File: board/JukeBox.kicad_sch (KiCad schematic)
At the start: 44 parts, among them J1 USB_C_Receptacle_USB2.0, J2 Conn_01x02, J3 Conn_01x04, J4 Conn_01x03, J5 Conn_01x08, SW1 SW_SPST, SW10 SW_SPST, SW11 SW_SPST, SW12 SW_SPST, SW2 SW_SPST, SW3 SW_SPST, SW4 SW_SPST, SW5 SW_SPST, SW6 SW_SPST, SW7 SW_SPST, SW8 SW_SPST, SW9 SW_SPST, U1 ATmega8U2-A, Y1 16MHz

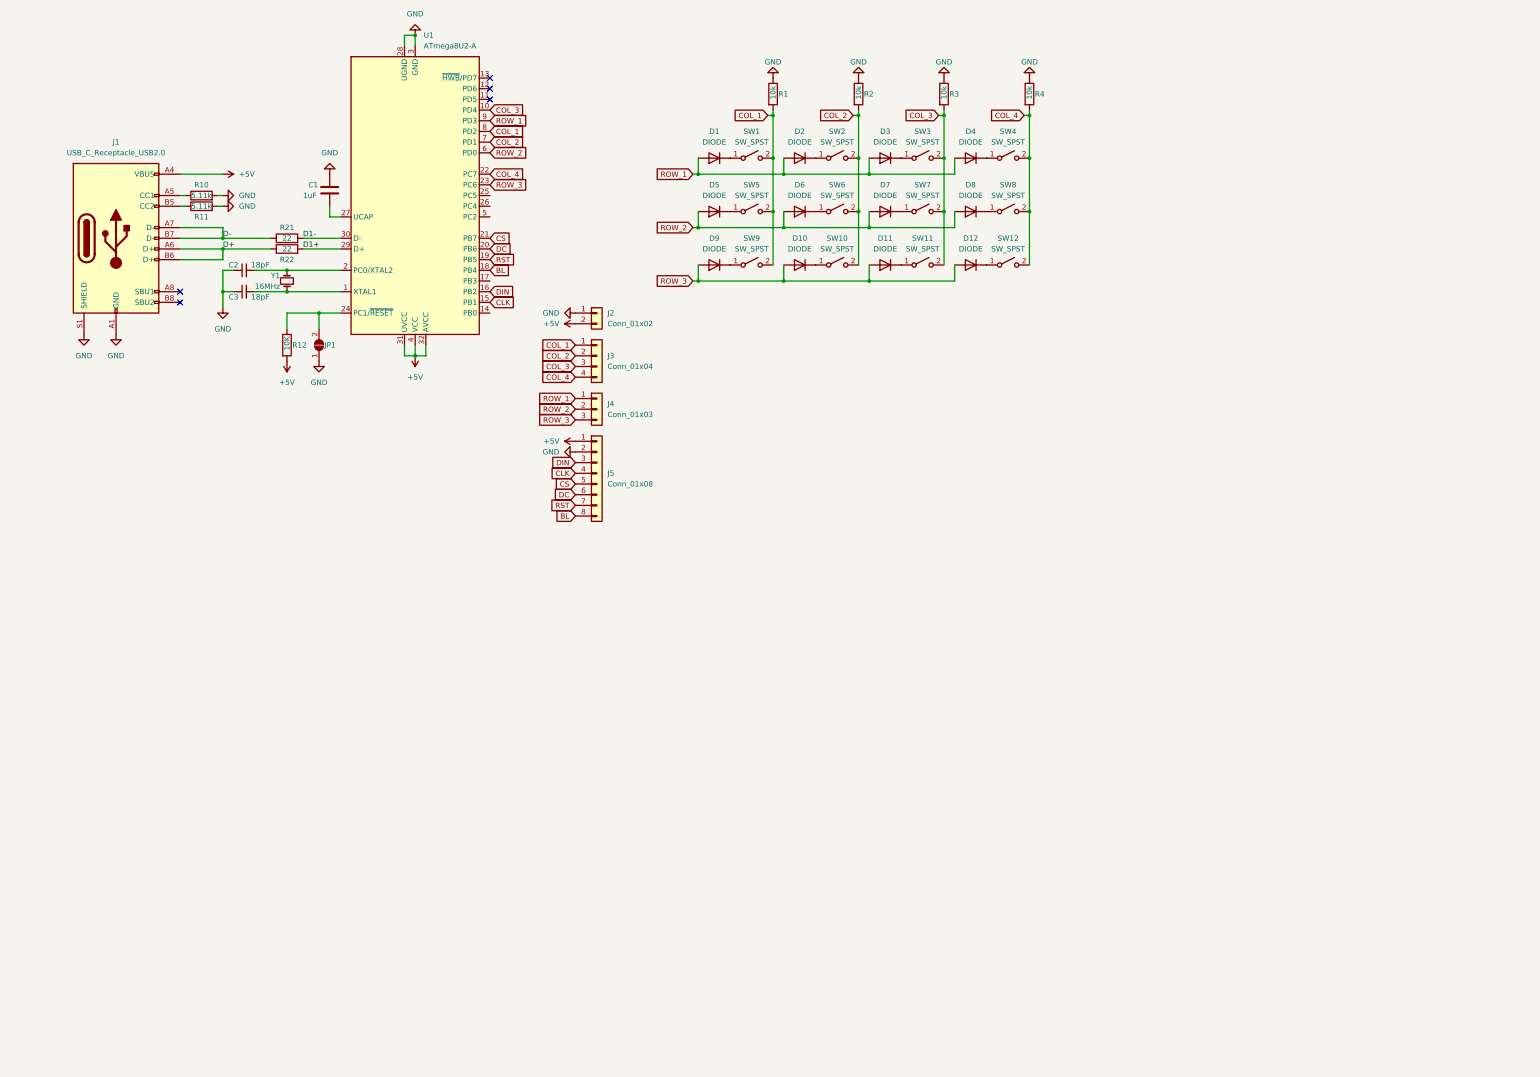
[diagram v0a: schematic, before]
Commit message: import rp2040 minimal kicad project
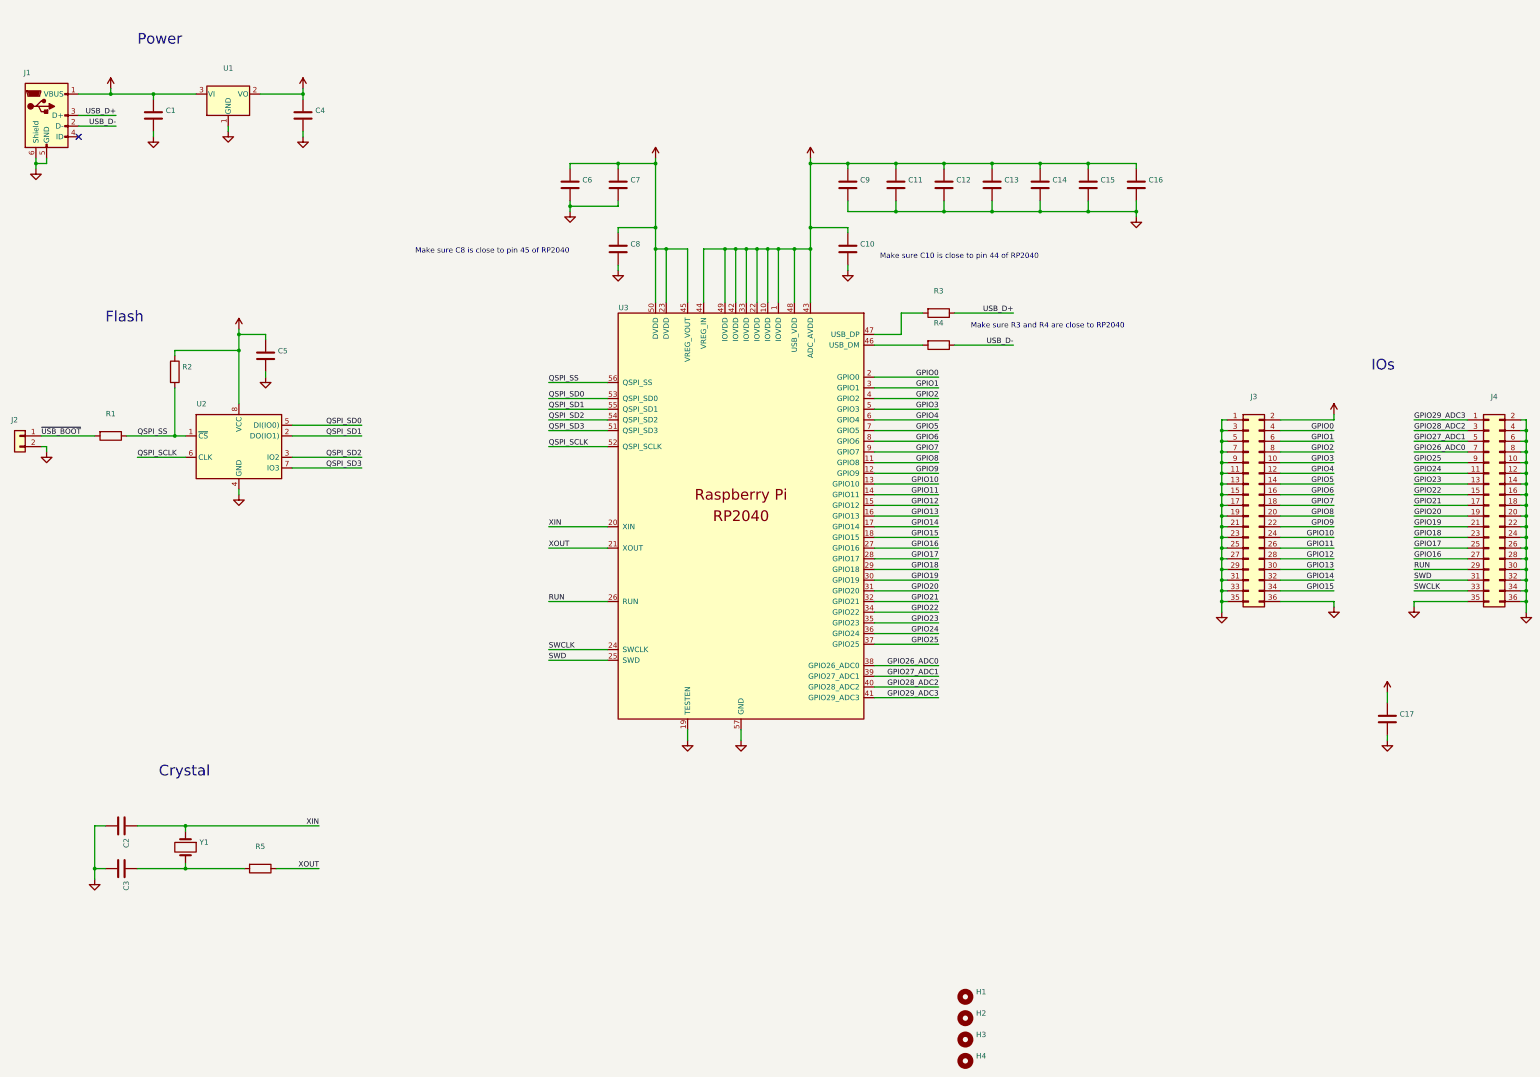
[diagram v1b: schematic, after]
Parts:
- removed C2, C3: 18pF, Capacitor_SMD:C_1206_3216Metric_Pad1.33x1.80mm_HandSolder, symbol Device:C_Small
- removed D1, D10, D11, D12, D2, D3, D4, D5, D6, D7, D8, D9: DIODE, Diode_SMD:D_1206_3216Metric_Pad1.42x1.75mm_HandSolder, symbol Simulation_SPICE:DIODE
- removed J1: USB_C_Receptacle_USB2.0, jukebox-footprints:GCT_USB4085-GF-A_REVA4, symbol Connector:USB_C_Receptacle_USB2.0
- removed J3: Conn_01x04, Connector_PinHeader_2.54mm:PinHeader_1x04_P2.54mm_Vertical, symbol Connector_Generic:Conn_01x04
- removed J4: Conn_01x03, Connector_PinHeader_2.54mm:PinHeader_1x03_P2.54mm_Vertical, symbol Connector_Generic:Conn_01x03
- removed J5: Conn_01x08, Connector_PinHeader_2.54mm:PinHeader_1x08_P2.54mm_Vertical, symbol Connector_Generic:Conn_01x08
- removed JP1: (no value), Jumper:SolderJumper-2_P1.3mm_Open_Pad1.0x1.5mm, symbol Jumper:SolderJumper_2_Open
- removed R10, R11: 5.11k, Resistor_SMD:R_1206_3216Metric_Pad1.30x1.75mm_HandSolder, symbol Device:R
- removed R12: 10K, Resistor_SMD:R_1206_3216Metric_Pad1.30x1.75mm_HandSolder, symbol Device:R
- removed R21, R22: 22, Resistor_SMD:R_1206_3216Metric_Pad1.30x1.75mm_HandSolder, symbol Device:R
- removed SW1, SW10, SW11, SW12, SW2, SW3, SW4, SW5, SW6, SW7, SW8, SW9: SW_SPST, jukebox-footprints:Kailh_PG1350, symbol Switch:SW_SPST
- removed U1: ATmega8U2-A, Package_QFP:TQFP-32_7x7mm_P0.8mm, symbol MCU_Microchip_ATmega:ATmega8U2-A
- removed Y1: 16MHz, Crystal:Crystal_HC49-4H_Vertical, symbol Device:Crystal_Small
- added C10, C11, C12, C13, C14, C15, C16, C17, C2, C3, C4, C5, C6, C7, C8, C9: (no value), symbol Device:C
- added H1, H2, H3, H4: (no value), symbol Mechanical:MountingHole
- added J1: (no value), symbol Connector:USB_B_Micro
- added J3, J4: (no value), symbol Connector_Generic:Conn_02x18_Odd_Even
- added R5: (no value), symbol Device:R
- added U1: (no value), symbol Regulator_Linear:NCP1117-3.3_SOT223
- added U2: (no value), symbol Memory_Flash:W25Q128JVS
- added U3: (no value), symbol MCU_RaspberryPi_RP2040:RP2040
- added Y1: (no value), symbol Device:Crystal
- C1: value 1uF -> (none); footprint Capacitor_SMD:C_1206_3216Metric_Pad1.33x1.80mm_HandSolder -> (none)
- J2: value Conn_01x02 -> (none); footprint Connector_PinHeader_2.54mm:PinHeader_1x02_P2.54mm_Vertical -> (none)
- R1, R2, R3, R4: value 10k -> (none); footprint Resistor_SMD:R_1206_3216Metric_Pad1.30x1.75mm_HandSolder -> (none)
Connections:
- net +5V is gone; now on net GND: J2.2 (Pin_2)
- net GND: now also C1.2, C10.2, C11.2, C12.2, C13.2, C14.2, C15.2, C16.2, C17.2, C2.2, C3.2, C4.2, C5.2, C6.2, C7.2, C8.2, C9.2, J1.5 (GND), J1.6 (Shield), J3.1 (Pin_1), J3.11 (Pin_11), J3.13 (Pin_13), J3.15 (Pin_15), J3.17 (Pin_17), J3.19 (Pin_19), J3.21 (Pin_21), J3.23 (Pin_23), J3.25 (Pin_25), J3.27 (Pin_27), J3.29 (Pin_29), J3.3 (Pin_3), J3.31 (Pin_31), J3.33 (Pin_33), J3.35 (Pin_35), J3.36 (Pin_36), J3.5 (Pin_5), J3.7 (Pin_7), J3.9 (Pin_9), J4.10 (Pin_10), J4.12 (Pin_12), J4.14 (Pin_14), J4.16 (Pin_16), J4.18 (Pin_18), J4.2 (Pin_2), J4.20 (Pin_20), J4.22 (Pin_22), J4.24 (Pin_24), J4.26 (Pin_26), J4.28 (Pin_28), J4.30 (Pin_30), J4.32 (Pin_32), J4.34 (Pin_34), J4.35 (Pin_35), J4.36 (Pin_36), J4.4 (Pin_4), J4.6 (Pin_6), J4.8 (Pin_8), U1.1 (GND), U2.4 (GND), U3.19 (TESTEN), U3.57 (GND); no longer C1.1, J2.1 (Pin_1), R1.1, R2.1, R3.1, R4.1
- net COL_1 renamed ~{USB_BOOT}
- net ~{USB_BOOT}: now also J2.1 (Pin_1)
- net COL_2 renamed QSPI_SS
- net QSPI_SS: now also R1.1, U2.1 (~{CS}), U3.56 (QSPI_SS)
- net COL_3: no longer names the net of R3.2
- net COL_3: now also U3.47 (USB_DP)
- net COL_4: no longer names the net of R4.2
- net COL_4: now also U3.46 (USB_DM)
- new net: C3.1, R5.2, Y1.2
- new net +1V1: C6.1, C7.1, C8.1, U3.23 (DVDD), U3.45 (VREG_VOUT), U3.50 (DVDD)
- new net +3V3: C10.1, C11.1, C12.1, C13.1, C14.1, C15.1, C16.1, C17.1, C4.1, C5.1, C9.1, J3.2 (Pin_2), R2.1, U1.2 (VO), U2.8 (VCC), U3.1 (IOVDD), U3.10 (IOVDD), U3.22 (IOVDD), U3.33 (IOVDD), U3.42 (IOVDD), U3.43 (ADC_AVDD), U3.44 (VREG_IN), U3.48 (USB_VDD), U3.49 (IOVDD)
- new net GPIO0: J3.4 (Pin_4), U3.2 (GPIO0)
- new net GPIO1: J3.6 (Pin_6), U3.3 (GPIO1)
- new net GPIO10: J3.24 (Pin_24), U3.13 (GPIO10)
- new net GPIO11: J3.26 (Pin_26), U3.14 (GPIO11)
- new net GPIO12: J3.28 (Pin_28), U3.15 (GPIO12)
- new net GPIO13: J3.30 (Pin_30), U3.16 (GPIO13)
- new net GPIO14: J3.32 (Pin_32), U3.17 (GPIO14)
- new net GPIO15: J3.34 (Pin_34), U3.18 (GPIO15)
- new net GPIO16: J4.27 (Pin_27), U3.27 (GPIO16)
- new net GPIO17: J4.25 (Pin_25), U3.28 (GPIO17)
- new net GPIO18: J4.23 (Pin_23), U3.29 (GPIO18)
- new net GPIO19: J4.21 (Pin_21), U3.30 (GPIO19)
- new net GPIO2: J3.8 (Pin_8), U3.4 (GPIO2)
- new net GPIO20: J4.19 (Pin_19), U3.31 (GPIO20)
- new net GPIO21: J4.17 (Pin_17), U3.32 (GPIO21)
- new net GPIO22: J4.15 (Pin_15), U3.34 (GPIO22)
- new net GPIO23: J4.13 (Pin_13), U3.35 (GPIO23)
- new net GPIO24: J4.11 (Pin_11), U3.36 (GPIO24)
- new net GPIO25: J4.9 (Pin_9), U3.37 (GPIO25)
- new net GPIO26_ADC0: J4.7 (Pin_7), U3.38 (GPIO26_ADC0)
- new net GPIO27_ADC1: J4.5 (Pin_5), U3.39 (GPIO27_ADC1)
- new net GPIO28_ADC2: J4.3 (Pin_3), U3.40 (GPIO28_ADC2)
- new net GPIO29_ADC3: J4.1 (Pin_1), U3.41 (GPIO29_ADC3)
- new net GPIO3: J3.10 (Pin_10), U3.5 (GPIO3)
- new net GPIO4: J3.12 (Pin_12), U3.6 (GPIO4)
- new net GPIO5: J3.14 (Pin_14), U3.7 (GPIO5)
- new net GPIO6: J3.16 (Pin_16), U3.8 (GPIO6)
- new net GPIO7: J3.18 (Pin_18), U3.9 (GPIO7)
- new net GPIO8: J3.20 (Pin_20), U3.11 (GPIO8)
- new net GPIO9: J3.22 (Pin_22), U3.12 (GPIO9)
- new net QSPI_SCLK: U2.6 (CLK), U3.52 (QSPI_SCLK)
- new net QSPI_SD0: U2.5 (DI(IO0)), U3.53 (QSPI_SD0)
- new net QSPI_SD1: U2.2 (DO(IO1)), U3.55 (QSPI_SD1)
- new net QSPI_SD2: U2.3 (IO2), U3.54 (QSPI_SD2)
- new net QSPI_SD3: U2.7 (IO3), U3.51 (QSPI_SD3)
- new net RUN: J4.29 (Pin_29), U3.26 (RUN)
- new net SWCLK: J4.33 (Pin_33), U3.24 (SWCLK)
- new net SWD: J4.31 (Pin_31), U3.25 (SWD)
- new net USB_D+: J1.3 (D+), R3.1
- new net USB_D-: J1.2 (D-), R4.1
- new net VBUS: C1.1, J1.1 (VBUS), U1.3 (VI)
- new net XIN: C2.1, U3.20 (XIN), Y1.1
- new net XOUT: R5.1, U3.21 (XOUT)
- no-connect marks 5 -> 1
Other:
- note added: "Crystal"
- note added: "Flash"
- note added: "IOs"
- note added: "Make sure C10 is close to pin 44 of RP2040"
- note added: "Make sure C8 is close to pin 45 of RP2040"
- note added: "Make sure R3 and R4 are close to RP2040"
- note added: "Power"
- company: (none) -> Raspberry Pi (Trading) Ltd
- title: (none) -> RP2040 Minimal Design Example
